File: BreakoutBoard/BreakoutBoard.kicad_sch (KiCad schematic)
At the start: 21 parts, among them J1 QTE-020-01-X-D-A, J10 Conn_01x01_Female, J11 SBH11-NBPC-D12-SM-BK, J2 QTE-020-01-X-D-A, J3 Conn_01x01_Female, J4 Conn_01x01_Female, J5 Conn_01x01_Female, J6 Conn_01x01_Female, J7 Conn_01x01_Female, J8 Conn_01x01_Female, J9 Conn_01x01_Female, Q1 STB40N60M2

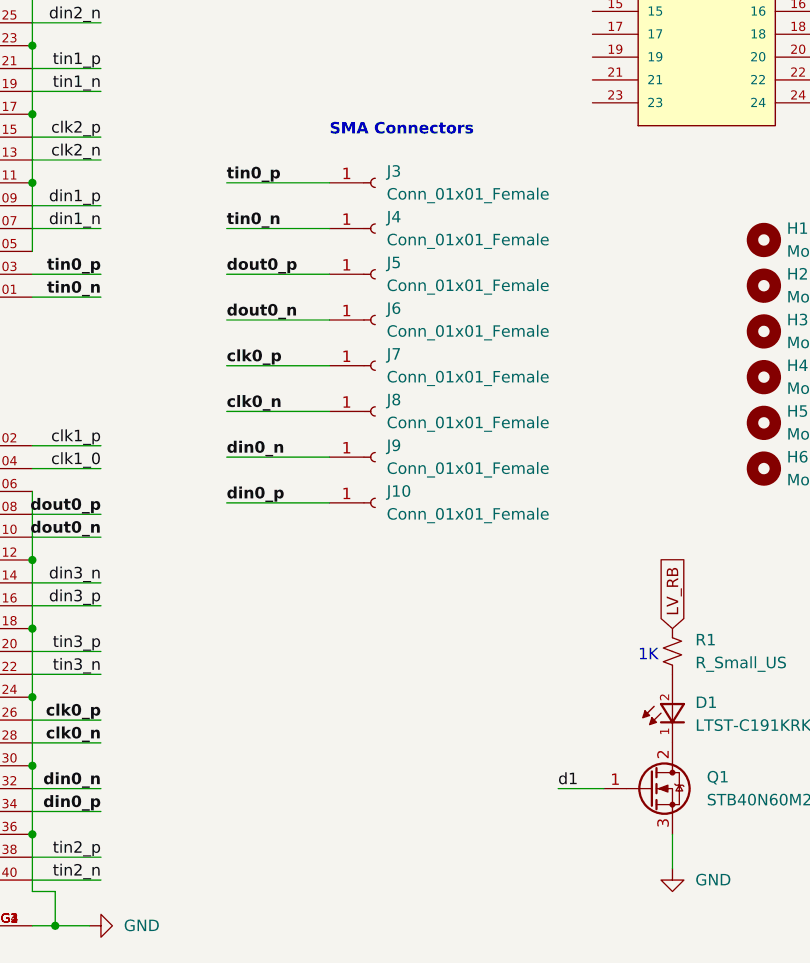
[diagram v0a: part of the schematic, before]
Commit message: Fixed issues
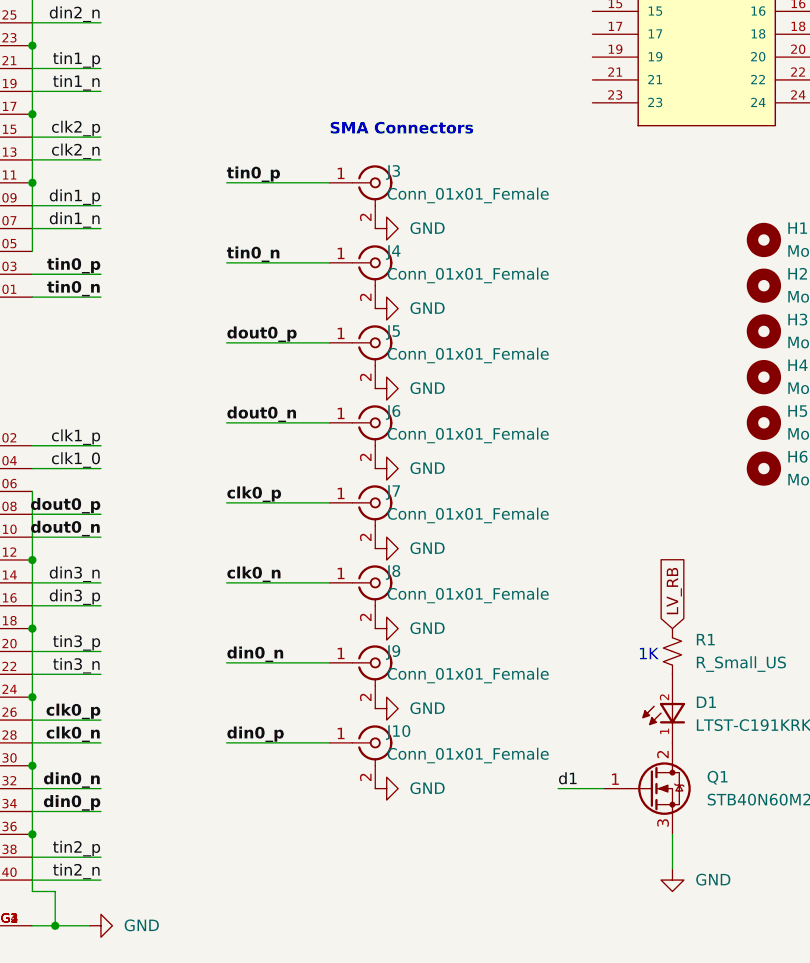
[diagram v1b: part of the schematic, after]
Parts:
- J10, J3, J4, J5, J6, J7, J8, J9: symbol Connector:Conn_01x01_Female -> Connector:Conn_Coaxial
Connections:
- net GND: now also J10.2 (Ext), J3.2 (Ext), J4.2 (Ext), J5.2 (Ext), J6.2 (Ext), J7.2 (Ext), J8.2 (Ext), J9.2 (Ext)
